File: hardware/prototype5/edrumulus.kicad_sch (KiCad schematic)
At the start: 67 parts, among them J1 Trigger Connector, J2 Raspberry Pi GPIO pins, U1 ESP32-WROOM-32U

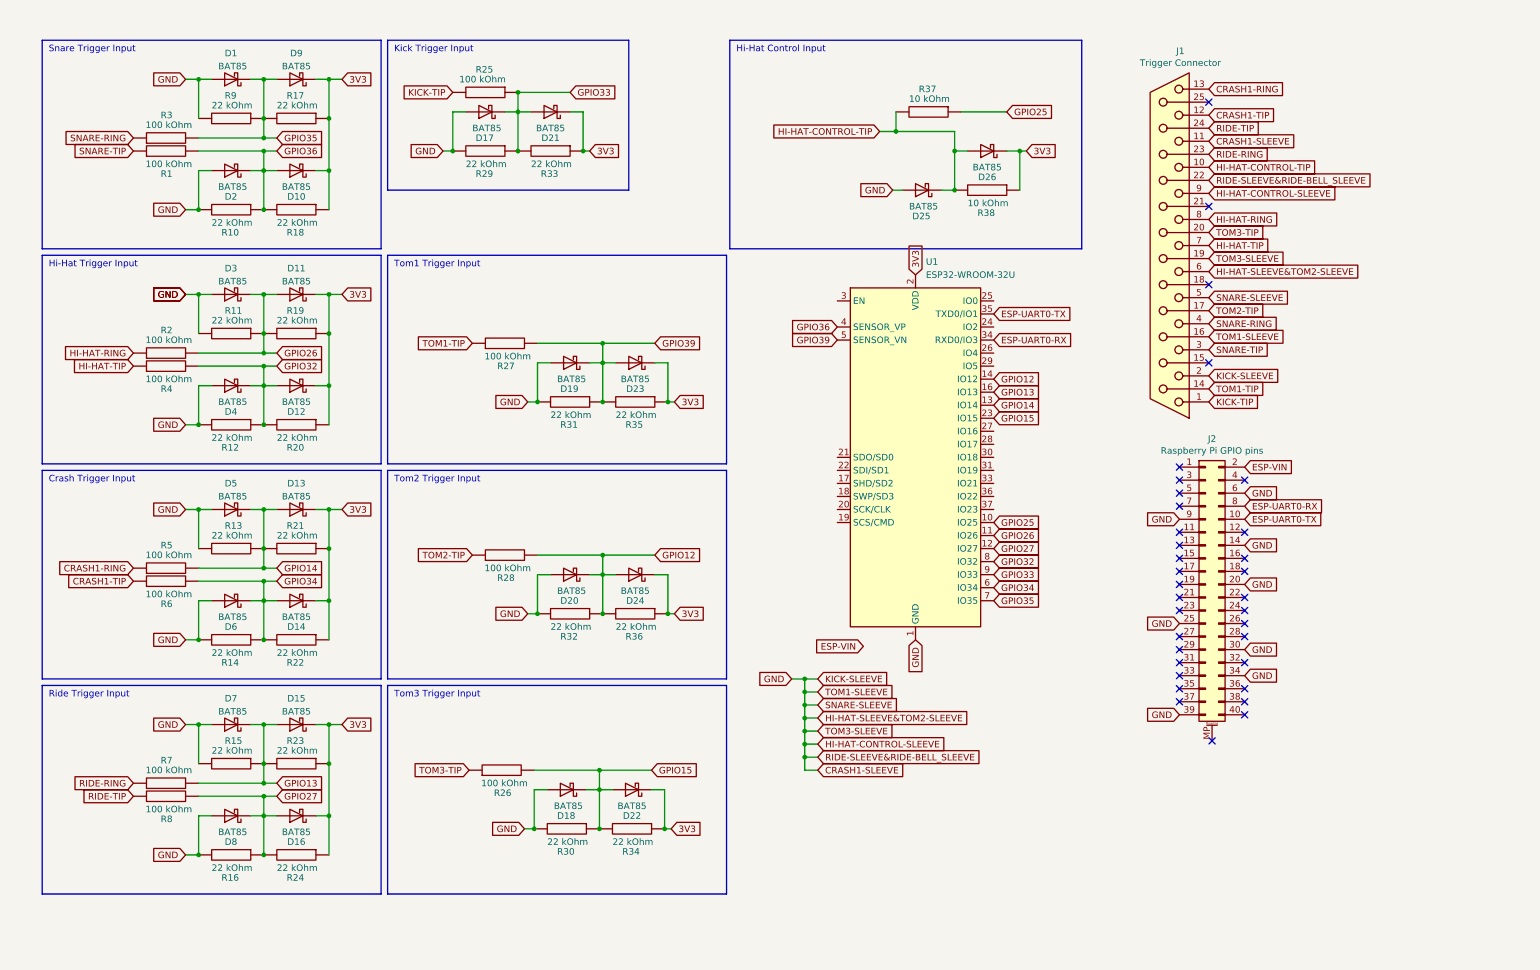
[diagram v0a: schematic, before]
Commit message: some more work for prototype 5
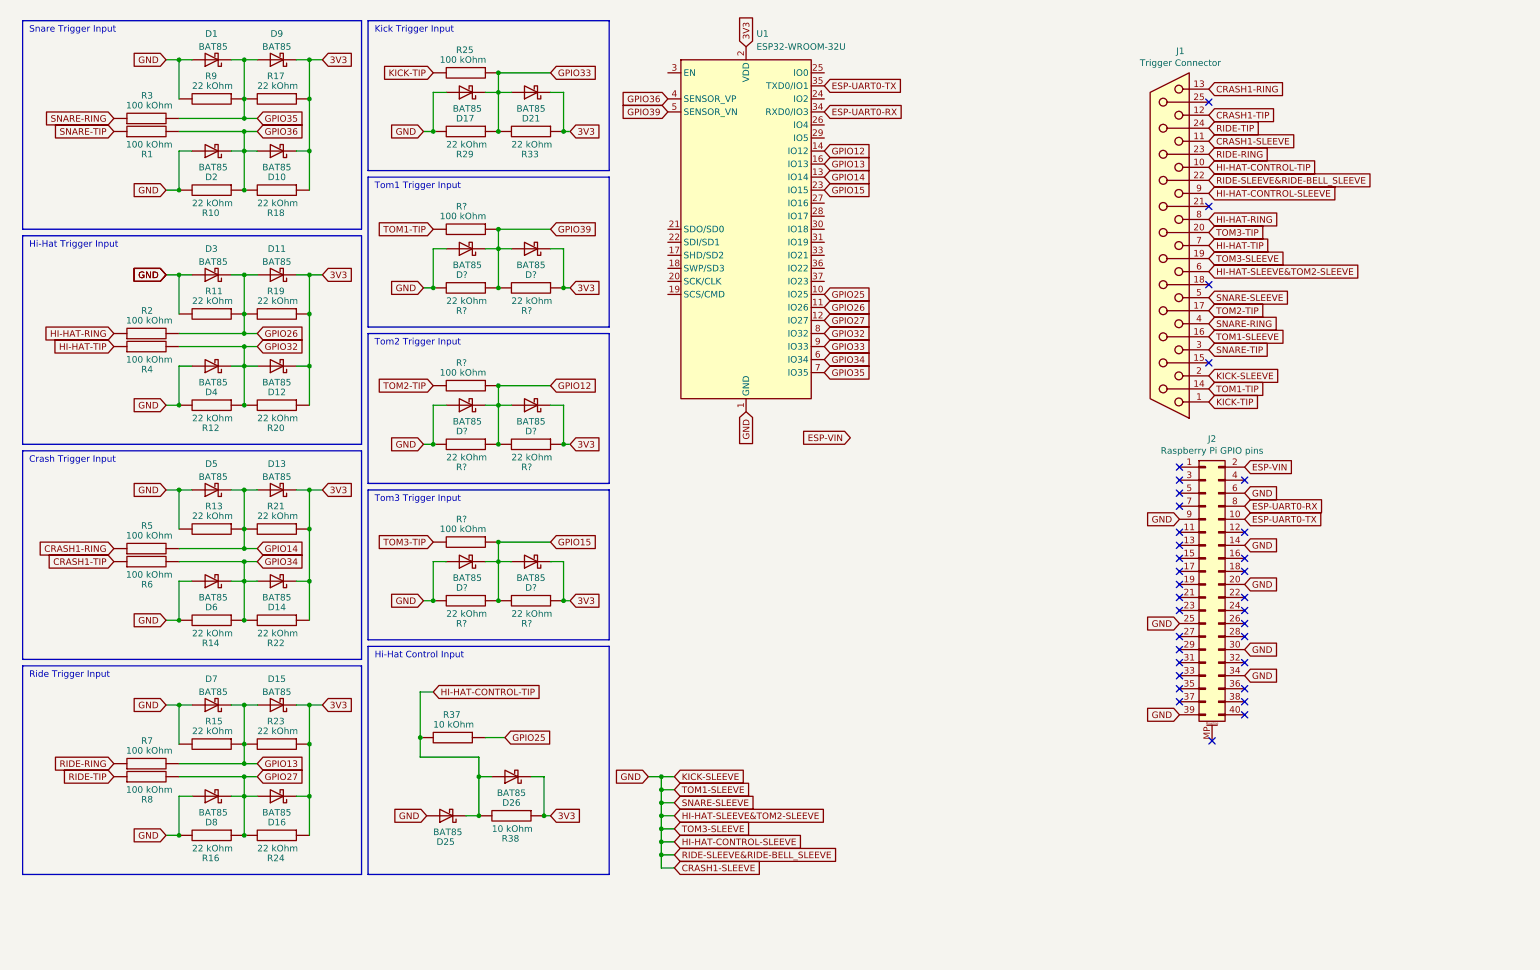
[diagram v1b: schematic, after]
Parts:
- removed D18, D19, D20, D22, D23, D24: BAT85, Diode_SMD:D_MiniMELF, symbol Diode:BAT85
- removed R26, R27, R28: 100 kOhm, Resistor_SMD:R_1206_3216Metric_Pad1.30x1.75mm_HandSolder, symbol pspice:R
- removed R30, R31, R32, R34, R35, R36: 22 kOhm, Resistor_SMD:R_1206_3216Metric_Pad1.30x1.75mm_HandSolder, symbol pspice:R
- added D? (x6): BAT85, Diode_SMD:D_MiniMELF, symbol Diode:BAT85
- added R? (x6): 22 kOhm, Resistor_SMD:R_1206_3216Metric_Pad1.30x1.75mm_HandSolder, symbol pspice:R
- added R? (x3): 100 kOhm, Resistor_SMD:R_1206_3216Metric_Pad1.30x1.75mm_HandSolder, symbol pspice:R
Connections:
- net 3V3: now also D?.1 (K), D?.1 (K), D?.1 (K), R?.1, R?.1, R?.1
- net CRASH1-SLEEVE: now also D?.2 (A), D?.2 (A), D?.2 (A), R?.2, R?.2, R?.2
- net GPIO12: now also D?.1 (K), D?.2 (A), R?.1, R?.1, R?.2
- net GPIO15: now also D?.1 (K), D?.2 (A), R?.1, R?.1, R?.2
- net GPIO39: now also D?.1 (K), D?.2 (A), R?.1, R?.1, R?.2
- net TOM1-TIP: now also R?.2
- net TOM2-TIP: now also R?.2
- net TOM3-TIP: now also R?.2
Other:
- moved on the sheet: D1, D10, D11, D12, D13, D14, D15, D16, D17, D2, D21, D25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

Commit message: some more work on prototype 5
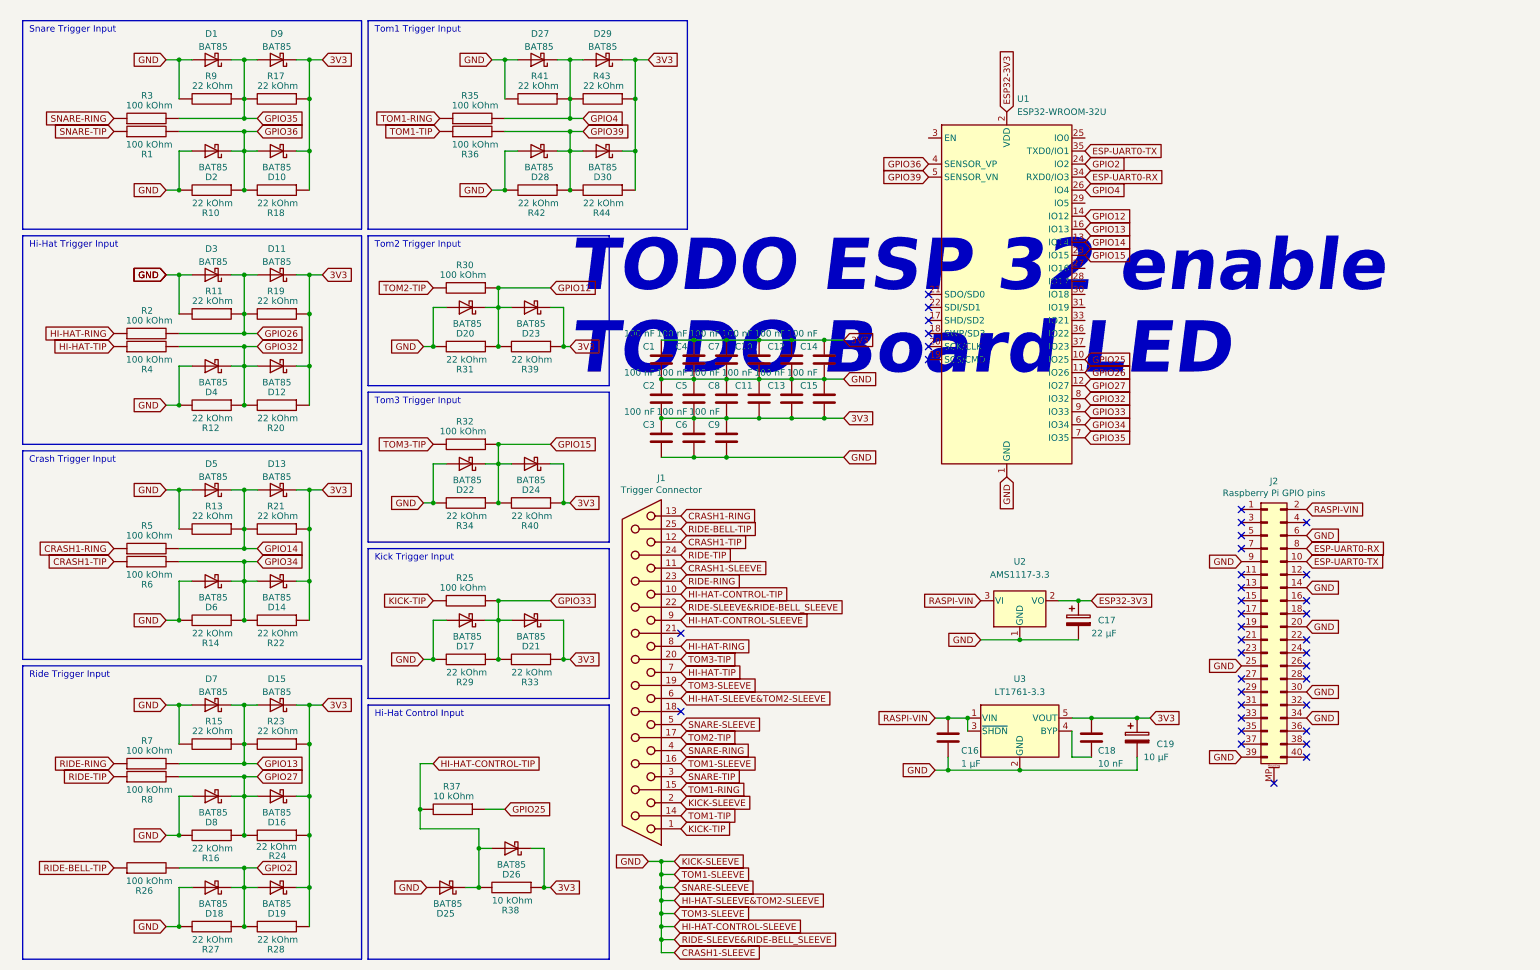
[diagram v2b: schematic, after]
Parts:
- removed D? (x2): BAT85, Diode_SMD:D_MiniMELF, symbol Diode:BAT85
- removed R? (x2): 22 kOhm, Resistor_SMD:R_1206_3216Metric_Pad1.30x1.75mm_HandSolder, symbol pspice:R
- removed R?: 100 kOhm, Resistor_SMD:R_1206_3216Metric_Pad1.30x1.75mm_HandSolder, symbol pspice:R
- added C1, C10, C11, C12, C13, C14, C15, C2, C3, C4, C5, C6, C7, C8, C9: 100 nF, symbol Device:C
- added C16: 1 µF, symbol Device:C
- added C17: 22 µF, symbol Device:C_Polarized
- added C18: 10 nF, symbol Device:C
- added C19: 10 µF, symbol Device:C_Polarized
- added D18, D19, D27, D28, D29, D30: BAT85, Diode_SMD:D_MiniMELF, symbol Diode:BAT85
- added R26, R35, R36: 100 kOhm, Resistor_SMD:R_1206_3216Metric_Pad1.30x1.75mm_HandSolder, symbol pspice:R
- added R27, R28, R41, R42, R43, R44: 22 kOhm, Resistor_SMD:R_1206_3216Metric_Pad1.30x1.75mm_HandSolder, symbol pspice:R
- added U2: AMS1117-3.3, Package_TO_SOT_SMD:SOT-223-3_TabPin2, symbol Regulator_Linear:AMS1117-3.3
- added U3: LT1761-3.3, Package_TO_SOT_SMD:TSOT-23-5, symbol Regulator_Linear:LT1761-3.3
- gave numbers to parts that had none: 10
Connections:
- net 3V3: now also C1.2, C10.2, C11.1, C12.2, C13.1, C14.2, C15.1, C18.1, C19.1, C2.1, C3.2, C4.2, C5.1, C6.2, C7.2, C8.1, C9.2, D19.1 (K), D29.1 (K), D30.1 (K), R28.1, R43.1, R44.1, U3.5 (VOUT); no longer U1.2 (VDD)
- net CRASH1-SLEEVE: now also C1.1, C10.1, C11.2, C12.1, C13.2, C14.1, C15.2, C16.2, C17.2, C19.2, C2.2, C3.1, C4.1, C5.2, C6.1, C7.1, C8.2, C9.1, D18.2 (A), D27.2 (A), D28.2 (A), R27.2, R41.2, R42.2, U2.1 (GND), U3.2 (GND)
- net GPIO39: now also D28.1 (K), D30.2 (A), R36.2, R42.1, R44.2
- net TOM1-TIP: now also R36.1
- net TOM1-RING: now reaches J1.15 (P15)
- net TOM1-RING: now also R35.1
- net RIDE-BELL-TIP: now reaches J1.25 (P25)
- net RIDE-BELL-TIP: now also R26.1
- net GPIO2: now reaches U1.24 (IO2)
- net GPIO2: now also D18.1 (K), D19.2 (A), R26.2, R27.1, R28.2
- net GPIO4: now reaches U1.26 (IO4)
- net GPIO4: now also D27.1 (K), D29.2 (A), R35.2, R41.1, R43.2
- net ESP-VIN renamed RASPI-VIN
- net RASPI-VIN: now also C16.1, U2.3 (VI), U3.1 (VIN), U3.3 (~{SHDN})
- new net: C18.2, U3.4 (BYP)
- new net ESP32-3V3: C17.1, U1.2 (VDD), U2.2 (VO)
- no-connect marks 34 -> 38
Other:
- note added: "TODO ESP 32 enable TODO Board LED"
- title: Edrumulus Prototype 4 (ESP32) -> Edrumulus Prototype 5 (ESP32)
- moved on the sheet: D17, D20, D21, D22, D23, D24, D25, D26, J1, J2, R25, R29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
